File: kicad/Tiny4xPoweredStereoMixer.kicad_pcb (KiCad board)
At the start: 4 copper layers, 83.9 x 66.9 mm, 0 parts

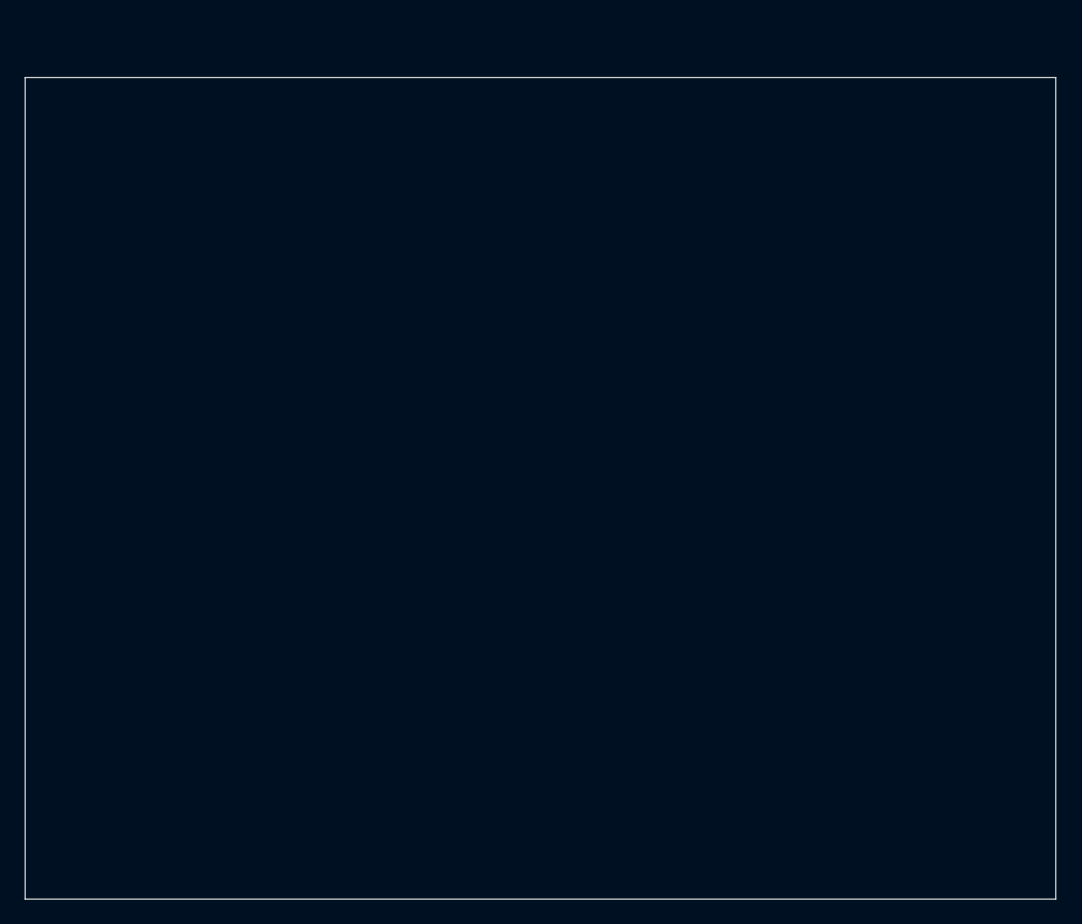
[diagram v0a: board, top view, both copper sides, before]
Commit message: Finished RevC layout
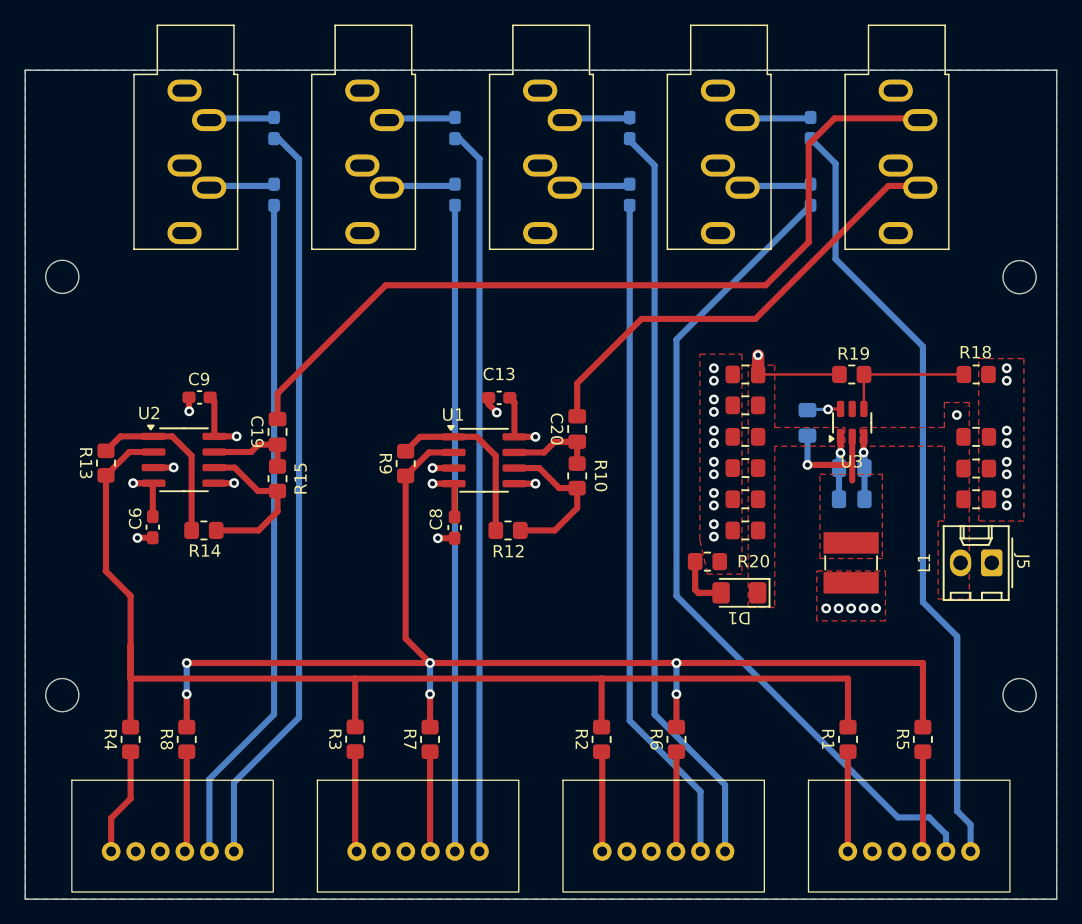
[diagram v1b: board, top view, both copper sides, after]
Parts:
- added C1: 10uF, Capacitor_SMD:C_0805_2012Metric_Pad1.18x1.45mm_HandSolder, F.Cu at (179.1, 80.0)
- added C10: 100nF, Capacitor_SMD:C_0603_1608Metric_Pad1.08x0.95mm_HandSolder, B.Cu at (136.7, 54.9)
- added C11: 100nF, Capacitor_SMD:C_0603_1608Metric_Pad1.08x0.95mm_HandSolder, B.Cu at (136.7, 60.3)
- added C12: 100nF, Capacitor_SMD:C_0603_1608Metric_Pad1.08x0.95mm_HandSolder, B.Cu at (150.9, 54.9)
- added C13: 100nF, Capacitor_SMD:C_0603_1608Metric_Pad1.08x0.95mm_HandSolder, F.Cu at (140.3, 76.8)
- added C14: 100nF, Capacitor_SMD:C_0603_1608Metric_Pad1.08x0.95mm_HandSolder, B.Cu at (150.9, 60.3)
- added C15: 10uF, Capacitor_SMD:C_0805_2012Metric_Pad1.18x1.45mm_HandSolder, B.Cu at (169.0, 82.5)
- added C16: 100nF, Capacitor_SMD:C_0805_2012Metric_Pad1.18x1.45mm_HandSolder, B.Cu at (165.4, 78.9)
- added C17: 100nF, Capacitor_SMD:C_0603_1608Metric_Pad1.08x0.95mm_HandSolder, B.Cu at (165.6, 54.9)
- added C18: 100nF, Capacitor_SMD:C_0603_1608Metric_Pad1.08x0.95mm_HandSolder, B.Cu at (165.6, 60.3)
- added C19: 10uF, Capacitor_SMD:C_0805_2012Metric_Pad1.18x1.45mm_HandSolder, F.Cu at (122.2, 79.6)
- added C2: 10uF, Capacitor_SMD:C_0805_2012Metric_Pad1.18x1.45mm_HandSolder, F.Cu at (179.1, 82.6)
- added C20: 10uF, Capacitor_SMD:C_0805_2012Metric_Pad1.18x1.45mm_HandSolder, F.Cu at (146.6, 79.4)
- added C21: 100nF, Capacitor_SMD:C_0805_2012Metric_Pad1.18x1.45mm_HandSolder, F.Cu at (160.3, 85.1)
- added C22: 22uF, Capacitor_SMD:C_0805_2012Metric_Pad1.18x1.45mm_HandSolder, F.Cu at (160.3, 87.6)
- added C23: 22uF, Capacitor_SMD:C_0805_2012Metric_Pad1.18x1.45mm_HandSolder, F.Cu at (160.3, 74.9)
- added C24: 22uF, Capacitor_SMD:C_0805_2012Metric_Pad1.18x1.45mm_HandSolder, F.Cu at (160.3, 77.4)
- added C25: 22uF, Capacitor_SMD:C_0805_2012Metric_Pad1.18x1.45mm_HandSolder, F.Cu at (160.3, 80.0)
- added C26: 22uF, Capacitor_SMD:C_0805_2012Metric_Pad1.18x1.45mm_HandSolder, F.Cu at (160.3, 82.5)
- added C3: 100nF, Capacitor_SMD:C_0805_2012Metric_Pad1.18x1.45mm_HandSolder, F.Cu at (179.1, 85.1)
- added C4: 100nF, Capacitor_SMD:C_0805_2012Metric_Pad1.18x1.45mm_HandSolder, B.Cu at (169.0, 85.1)
- added C5: 100nF, Capacitor_SMD:C_0603_1608Metric_Pad1.08x0.95mm_HandSolder, B.Cu at (121.9, 54.9)
- added C6: 100nF, Capacitor_SMD:C_0603_1608Metric_Pad1.08x0.95mm_HandSolder, F.Cu at (112.0, 87.4)
- added C7: 100nF, Capacitor_SMD:C_0603_1608Metric_Pad1.08x0.95mm_HandSolder, B.Cu at (121.9, 60.3)
- added C8: 100nF, Capacitor_SMD:C_0603_1608Metric_Pad1.08x0.95mm_HandSolder, F.Cu at (136.6, 87.4)
- added C9: 100nF, Capacitor_SMD:C_0603_1608Metric_Pad1.08x0.95mm_HandSolder, F.Cu at (115.9, 76.8)
- added D1: LED, LED_SMD:LED_1206_3216Metric_Pad1.42x1.75mm_HandSolder, F.Cu at (159.8, 92.7)
- added H1: MountingHole, MountingHole:MountingHole_2.7mm_M2.5, F.Cu at (104.7, 67.0)
- added H2: MountingHole, MountingHole:MountingHole_2.7mm_M2.5, F.Cu at (182.6, 67.0)
- added H3: MountingHole, MountingHole:MountingHole_2.7mm_M2.5, F.Cu at (104.7, 101.0)
- added H4: MountingHole, MountingHole:MountingHole_2.7mm_M2.5, F.Cu at (182.6, 101.0)
- added J1: AudioJack3_SwitchTR, Connector_Audio:Jack_3.5mm_CUI_SJ1-3535NG_Horizontal, F.Cu at (114.6, 51.8)
- added J2: AudioJack3_SwitchTR, Connector_Audio:Jack_3.5mm_CUI_SJ1-3535NG_Horizontal, F.Cu at (129.1, 51.8)
- added J3: AudioJack3_SwitchTR, Connector_Audio:Jack_3.5mm_CUI_SJ1-3535NG_Horizontal, F.Cu at (143.6, 51.8)
- added J4: AudioJack3_SwitchTR, Connector_Audio:Jack_3.5mm_CUI_SJ1-3535NG_Horizontal, F.Cu at (158.1, 51.8)
- added J5: PowerConnector, Connector_Molex:Molex_KK-254_AE-6410-02A_1x02_P2.54mm_Vertical, F.Cu at (180.4, 90.3)
- added J9: AudioJack3_SwitchTR, Connector_Audio:Jack_3.5mm_CUI_SJ1-3535NG_Horizontal, F.Cu at (172.5, 51.8)
- added L1: 22uH, Inductor_SMD:L_Ferrocore_DLG-0403, F.Cu at (168.9, 90.3)
- added R1: 10k, Resistor_SMD:R_0805_2012Metric_Pad1.20x1.40mm_HandSolder, F.Cu at (168.7, 104.6)
- added R10: 10k, Resistor_SMD:R_0805_2012Metric_Pad1.20x1.40mm_HandSolder, F.Cu at (146.6, 83.2)
- added R12: 10k, Resistor_SMD:R_0805_2012Metric_Pad1.20x1.40mm_HandSolder, F.Cu at (141.0, 87.6)
- added R13: 10k, Resistor_SMD:R_0805_2012Metric_Pad1.20x1.40mm_HandSolder, F.Cu at (108.2, 82.1)
- added R14: 10k, Resistor_SMD:R_0805_2012Metric_Pad1.20x1.40mm_HandSolder, F.Cu at (116.2, 87.6)
- added R15: 10k, Resistor_SMD:R_0805_2012Metric_Pad1.20x1.40mm_HandSolder, F.Cu at (122.2, 83.4)
- added R18: 50K, Resistor_SMD:R_0805_2012Metric_Pad1.20x1.40mm_HandSolder, F.Cu at (179.1, 74.9)
- added R19: 2K4, Resistor_SMD:R_0805_2012Metric_Pad1.20x1.40mm_HandSolder, F.Cu at (169.0, 74.9)
- added R2: 10k, Resistor_SMD:R_0805_2012Metric_Pad1.20x1.40mm_HandSolder, F.Cu at (148.6, 104.6)
- added R20: 2K2, Resistor_SMD:R_0805_2012Metric_Pad1.20x1.40mm_HandSolder, F.Cu at (157.2, 90.2)
- added R3: 10k, Resistor_SMD:R_0805_2012Metric_Pad1.20x1.40mm_HandSolder, F.Cu at (128.5, 104.6)
- added R4: 10k, Resistor_SMD:R_0805_2012Metric_Pad1.20x1.40mm_HandSolder, F.Cu at (110.2, 104.6)
- added R5: 10k, Resistor_SMD:R_0805_2012Metric_Pad1.20x1.40mm_HandSolder, F.Cu at (174.8, 104.6)
- added R6: 10k, Resistor_SMD:R_0805_2012Metric_Pad1.20x1.40mm_HandSolder, F.Cu at (154.7, 104.6)
- added R7: 10k, Resistor_SMD:R_0805_2012Metric_Pad1.20x1.40mm_HandSolder, F.Cu at (134.6, 104.6)
- added R8: 10k, Resistor_SMD:R_0805_2012Metric_Pad1.20x1.40mm_HandSolder, F.Cu at (114.8, 104.6)
- added R9: 10k, Resistor_SMD:R_0805_2012Metric_Pad1.20x1.40mm_HandSolder, F.Cu at (132.6, 82.2)
- added RV1: 10k, Potentiometers:Alps_RK12L12_Double_Horizontal, F.Cu at (113.7, 110.5)
- added RV2: 10k, Potentiometers:Alps_RK12L12_Double_Horizontal, F.Cu at (133.6, 110.5)
- added RV3: 10k, Potentiometers:Alps_RK12L12_Double_Horizontal, F.Cu at (153.6, 110.5)
- added RV4: 10k, Potentiometers:Alps_RK12L12_Double_Horizontal, F.Cu at (173.6, 110.5)
- added U1: TL072, Package_SO:SOIC-8_3.9x4.9mm_P1.27mm, F.Cu at (139.0, 81.9)
- added U2: TL072, Package_SO:SOIC-8_3.9x4.9mm_P1.27mm, F.Cu at (114.6, 81.9)
- added U3: TPS54202DDC, Package_TO_SOT_SMD:SOT-23-6, F.Cu at (169.0, 78.9)
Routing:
- net Net-(U1A--): track 0.00 -> 101.6 mm, vias 0 -> 6
- net Net-(U2A--): track 0.00 -> 98.9 mm
- net Net-(C19-Pad2): track 0.00 -> 68.4 mm
- net Net-(C18-Pad2): track 0.00 -> 68.1 mm
- net Net-(C17-Pad2): track 0.00 -> 63.8 mm
- net Net-(C5-Pad2): track 0.00 -> 61.6 mm
- net Net-(C12-Pad2): track 0.00 -> 61.6 mm
- net Net-(C10-Pad2): track 0.00 -> 59.4 mm
- net Net-(C14-Pad2): track 0.00 -> 55.4 mm
- net Net-(C7-Pad2): track 0.00 -> 54.8 mm
- net Net-(C11-Pad2): track 0.00 -> 52.8 mm
- net Net-(C20-Pad2): track 0.00 -> 37.3 mm
- net -12V: track 0.00 -> 22.2 mm, vias 0 -> 4
- net +12V: track 0.00 -> 15.3 mm, vias 0 -> 4
- net Net-(R12-Pad1): track 0.00 -> 14.5 mm
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- added copper zone on F.Cu, net +12V
- added copper zone on In1.Cu, net +12V
- added copper zone on F.Cu, net -12V
- added copper zone on In2.Cu, net -12V
- added copper zone on B.Cu, net GND
- added copper zone on F.Cu, net GND
- added copper zone on F.Cu, net Net-(U3-SW)
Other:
- board size 83.9 x 66.9 mm -> 84 x 67.5 mm
- board text added: "${PROJECTNAME}"
- board text added: "Rev ${REVISION} ${WEEK}"
